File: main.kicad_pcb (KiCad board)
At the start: 2 copper layers, 26 x 38 mm, 27 parts, among them J1 Screw_Terminal_01x02, M1 mDot, SW1 Reset, U1 BME280, U2 IRA-E700, U3 NCS36000

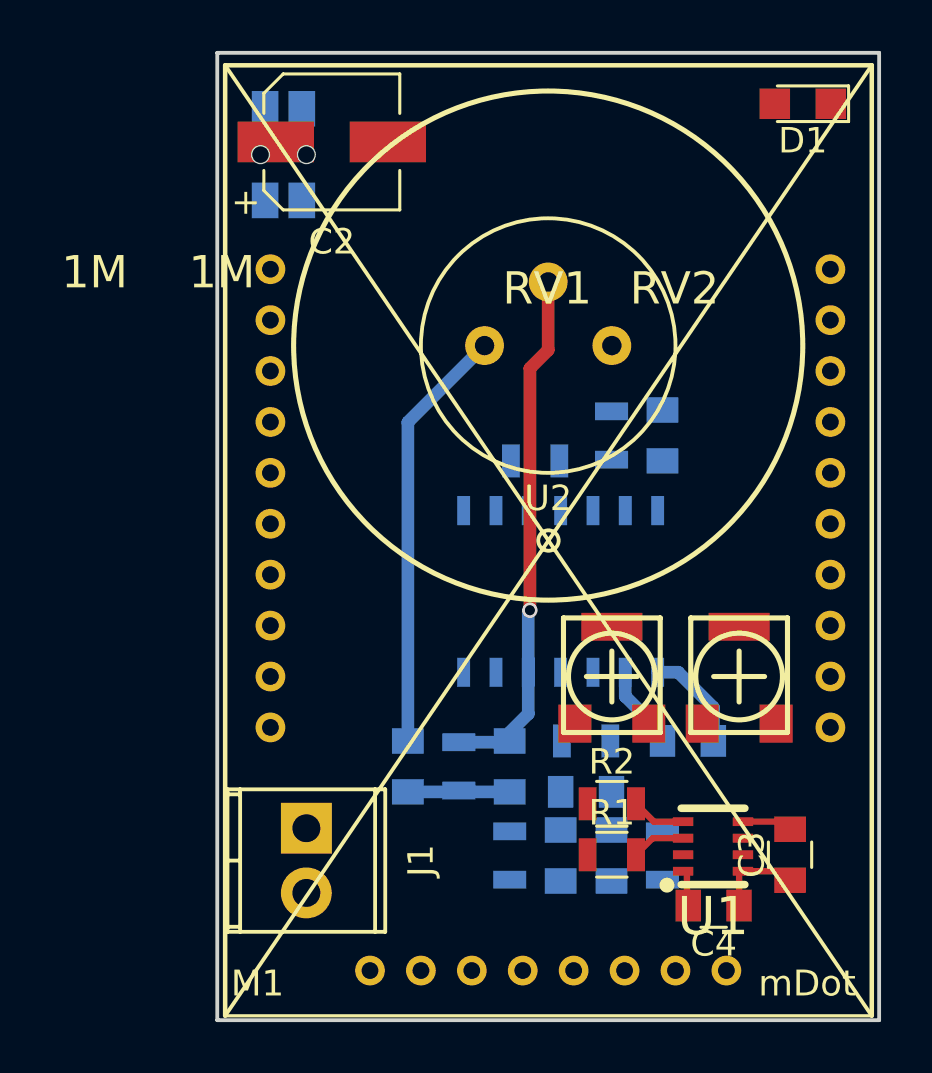
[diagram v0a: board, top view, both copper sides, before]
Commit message: test
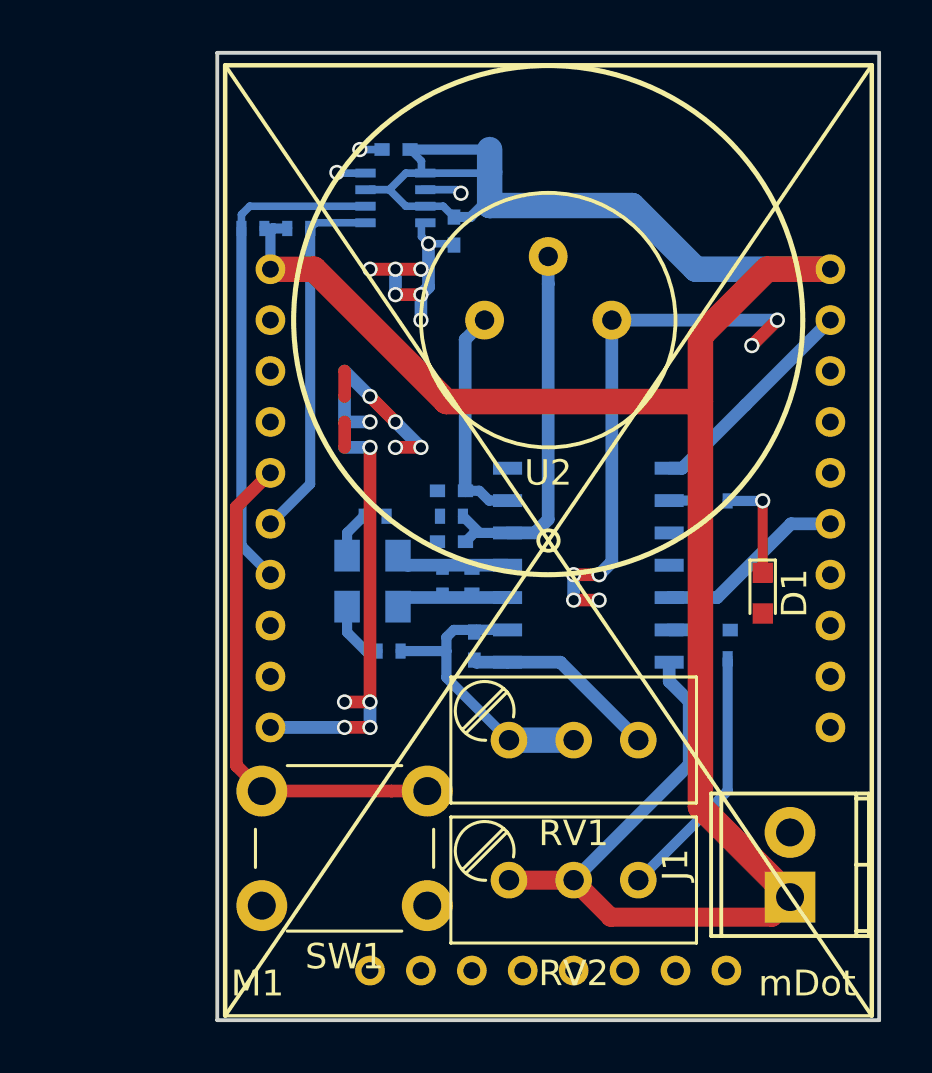
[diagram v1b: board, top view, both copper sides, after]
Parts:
- removed C2: 10µF, Capacitors_SMD:CP_Elec_5x4.5
- C1, C10, C7, C8, C9: footprint Capacitors_SMD:C_0805 -> Capacitors_SMD:C_0402
- C3, C4: footprint Capacitors_SMD:C_0805 -> Capacitors_SMD:C_0402; moved to B.Cu
- D1: footprint LEDs:LED_0805 -> LEDs:LED_0603
- R1, R2: footprint Resistors_SMD:R_0805 -> Resistors_SMD:R_0402; moved to B.Cu
- R3, R5, R6, R7, R8, R9: footprint Resistors_SMD:R_0805 -> Resistors_SMD:R_0402
- RV1, RV2: footprint STC:TRIM-EV1D-RMC -> Potentiometers:Potentiometer_Trimmer_Bourns_3296W
- SW1: footprint Buttons_Switches_SMD:SW_SPST_EVQP7C -> Buttons_Switches_THT:SW_PUSH_6mm_h5mm; moved to F.Cu
- U1: moved to B.Cu
- moved C4 32.2 mm to (199.0, 66.3)
- moved SW1 30.0 mm to (200.2, 96.0), turned to 180 degrees
- moved R1 28.4 mm to (193.4, 69.4), turned to 180 degrees
- moved C3 27.8 mm to (201.3, 69.5), turned to 270 degrees
- moved U1 26.1 mm to (200.2, 69.5)
- moved R2 25.7 mm to (195.2, 69.4)
- moved D1 19.3 mm to (213.4, 83.7), turned to 270 degrees
- moved J1 19.2 mm to (214.5, 95.7), turned to 90 degrees
- moved R5 14.3 mm to (198.2, 80.7), turned to 180 degrees
- moved C5 13.9 mm to (198.1, 82.3), turned to 0 degrees
- moved C6 13.6 mm to (198.1, 84.3), turned to 0 degrees
- moved R7 13.4 mm to (198.8, 86.0), turned to 180 degrees
- moved RV2 12.1 mm to (203.5, 95.0), turned to 180 degrees
- moved C9 11.0 mm to (201.2, 79.7), turned to 0 degrees
- moved C1 10.0 mm to (200.8, 83.3), turned to 270 degrees
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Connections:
- RV2 pad 1: Net-(R9-Pad2) -> +3V3
- RV2 pad 3: +3V3 -> Net-(R9-Pad2)
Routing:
- net +3V3: track 3.49 -> 104.5 mm
- net GND: track 7.49 -> 60.1 mm, vias 0 -> 26
- net Net-(M1-Pad5): track 0.00 -> 20.0 mm
- net Net-(M1-Pad7): track 2.27 -> 19.8 mm
- net Net-(M1-Pad6): track 2.29 -> 14.7 mm
- net Net-(R9-Pad2): track 0.00 -> 10.2 mm
- net Net-(C8-Pad2): track 3.30 -> 13.3 mm
- net Net-(M1-Pad19): track 0.00 -> 8.74 mm
- net Net-(C1-Pad2): track 0.00 -> 8.52 mm
- net Net-(C1-Pad1): track 0.00 -> 8.51 mm
- net Net-(C9-Pad2): track 16.8 -> 8.84 mm
- net Net-(M1-Pad15): track 0.00 -> 7.53 mm
- net Net-(C7-Pad2): track 20.7 -> 14.9 mm, vias 1 -> 0
- net Net-(D1-Pad1): track 0.00 -> 4.20 mm, vias 0 -> 1
- net Net-(C8-Pad1): track 4.15 -> 7.74 mm
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- added copper zone on F.Cu, net GND
